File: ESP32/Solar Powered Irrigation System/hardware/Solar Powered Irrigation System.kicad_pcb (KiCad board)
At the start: 2 copper layers, 91.6 x 57.8 mm, 75 parts, among them J1 PUMP, J11 INPUT, J15 BSEN, J2 SOIL SENSOR, J3 AM2301A, J4 OLED SCREEN, J5 Ultra Sonic, J7 USB_C Conn, M2 MountingHole_2.5mm_Pad, Q1 IRLML6344, Q2 IRLML6344, Q3 UMH3N, SW1 RotaryEncoder, SW2 RESET, SW3 FLASH, U1 AMS1117-3.3, U2 ESP32-WROOM, U3 LM2596S-3.3V, U4 LM2596S-3.3V, U5 CH340C, Y1 12MHz

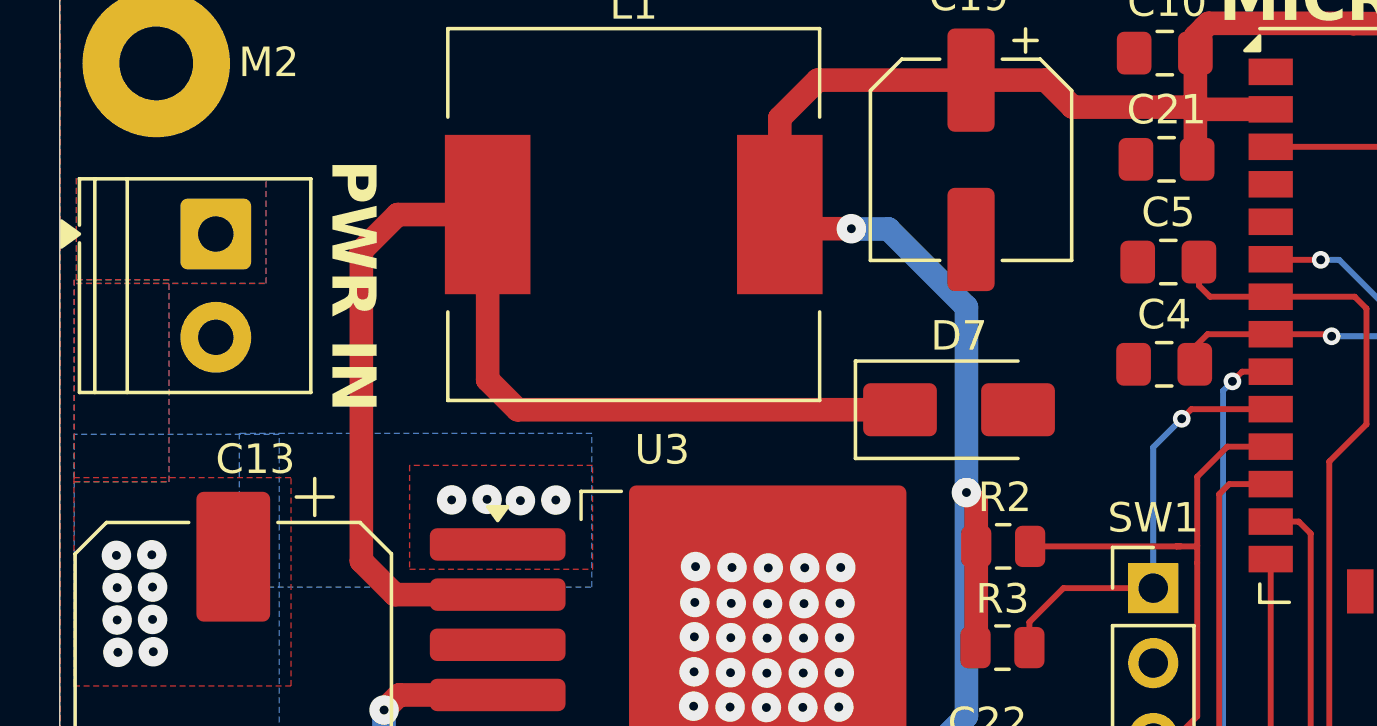
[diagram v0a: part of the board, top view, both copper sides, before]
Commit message: UPDATE FROM WORK
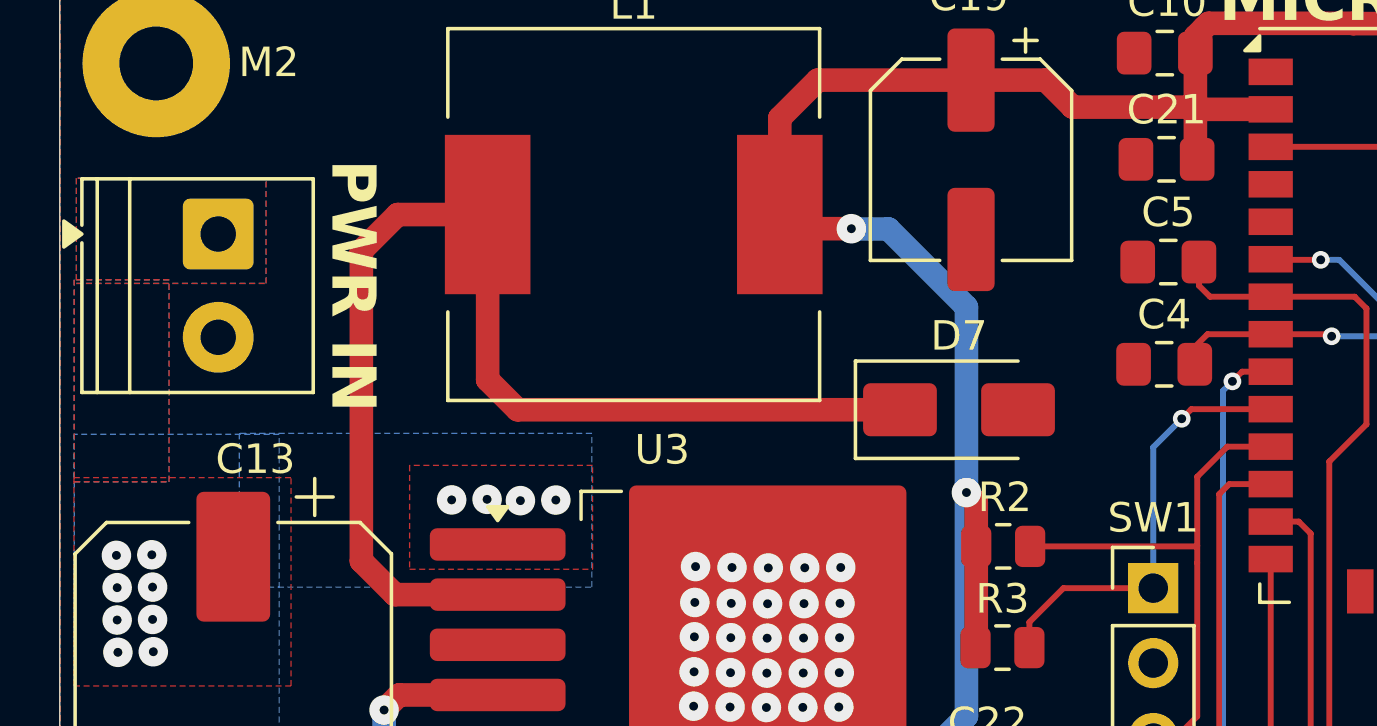
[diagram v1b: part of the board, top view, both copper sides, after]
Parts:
- moved J11 0.08 mm to (103.5, 88.3)
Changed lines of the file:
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@@
 	(footprint "TerminalBlock_Phoenix:TerminalBlock_Phoenix_PT-1,5-2-3.5-H_1x02_P3.50mm_Horizontal"
 		(layer "F.Cu")
-		(at 103.4025 88.29 -90)
+		(at 103.485 88.29 -90)
 		(descr "Terminal Block Phoenix PT-1,5-2-3.5-H, 2 pins, pitch 3.5mm, size 7x7.6mm, drill diameter 1.2mm, pad diameter 2.4mm, script-generated using https://gitlab.com/kicad/libraries/kicad-footprint-generator/-/tree/master/scripts/TerminalBlock_Phoenix")
 		(tags "THT Terminal Block Phoenix PT-1,5-2-3.5-H pitch 3.5mm size 7x7.6mm drill 1.2mm pad 2.4mm")
@@
 	)
 	(segment
-		(start 135.955 98.875)
+		(start 130.9975 98.875)
 		(end 136.64 98.875)
 		(width 0.2)
@@
 	)
 	(segment
-		(start 136.64 98.875)
-		(end 136.66 98.855)
-		(width 0.2)
-		(layer "F.Cu")
-		(net 36)
-	)
-	(segment
 		(start 135.925 105.37)
 		(end 136.66 104.635)
@@
 	)
 	(segment
-		(start 130.9975 98.875)
-		(end 135.955 98.875)
-		(width 0.2)
-		(layer "F.Cu")
-		(net 36)
-	)
-	(segment
 		(start 136.66 98.855)
 		(end 136.66 99.435)
@@
 	)
 	(segment
-		(start 135.955 98.875)
-		(end 136.1 98.875)
+		(start 136.64 98.875)
+		(end 136.66 98.855)
 		(width 0.2)
 		(layer "F.Cu")
@@
 		(layers "F.Cu" "B.Cu")
 		(hatch none 0.5)
-		(priority 1)
+		(priority 3)
 		(connect_pads yes
 			(clearance 0.3)
@@
 		(layer "B.Cu")
 		(hatch none 0.5)
-		(priority 1)
+		(priority 5)
 		(connect_pads yes
 			(clearance 0.3)
@@
 		(layer "B.Cu")
 		(hatch none 0.5)
-		(priority 1)
+		(priority 4)
 		(connect_pads yes
 			(clearance 0.3)
